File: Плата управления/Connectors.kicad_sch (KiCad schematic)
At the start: 9 parts, among them J1 Conn_02x10_Odd_Even, J11 Conn_02x07_Odd_Even, J2 CAN2, J3 CAN1, J4 A, J5 B, J6 C, J7 RS-485, J9 Conn_01x06

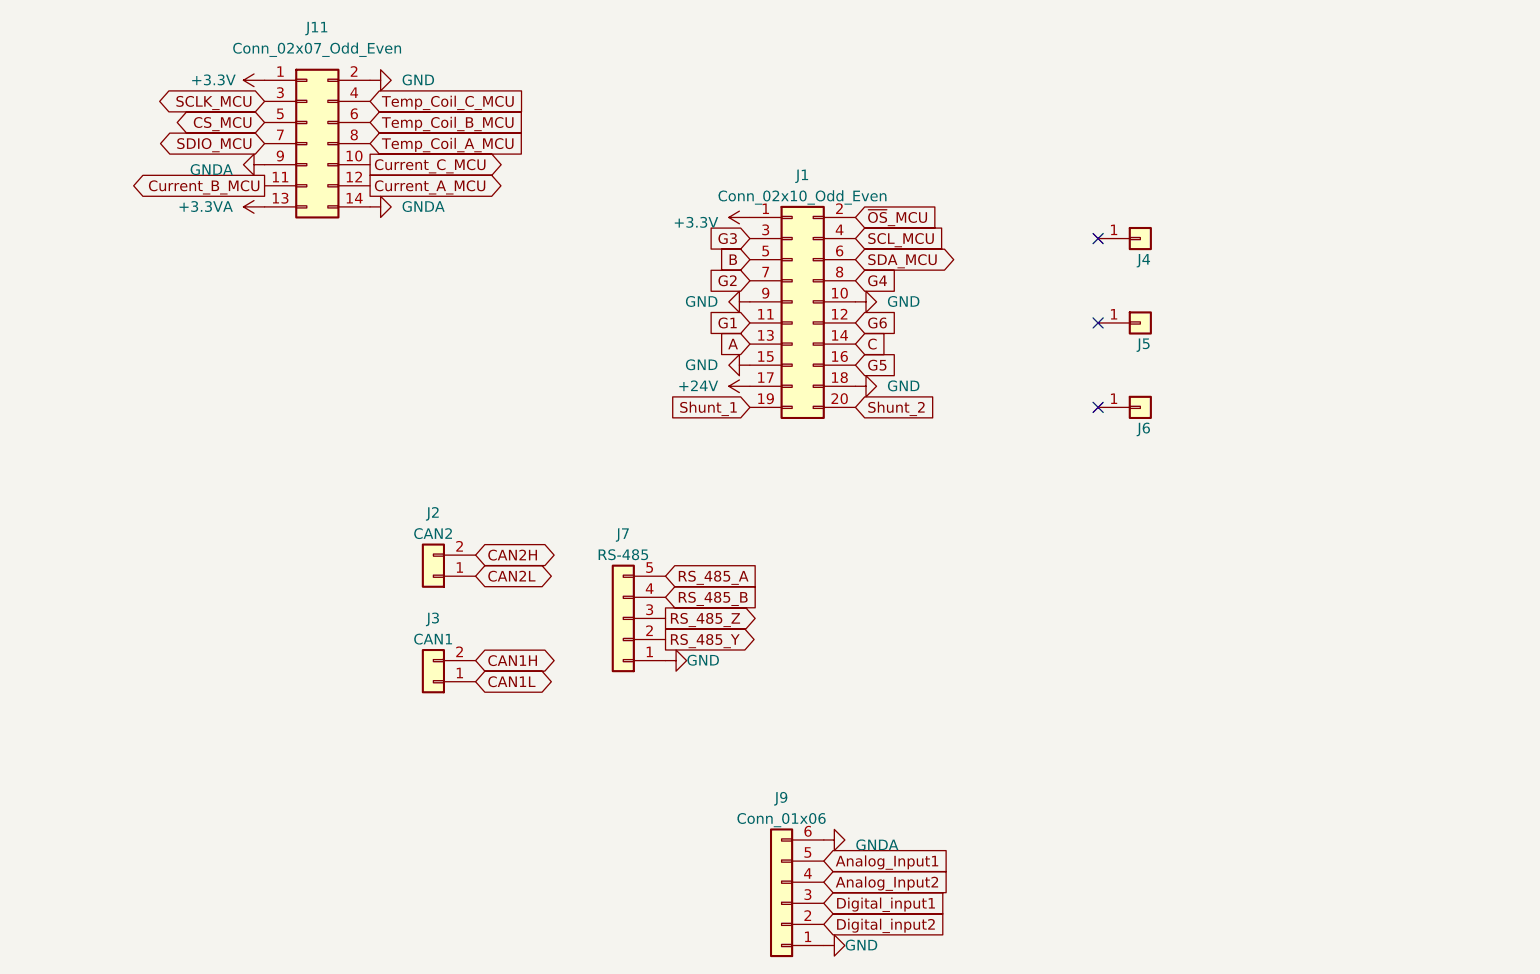
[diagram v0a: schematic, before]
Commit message: Редактировал схему
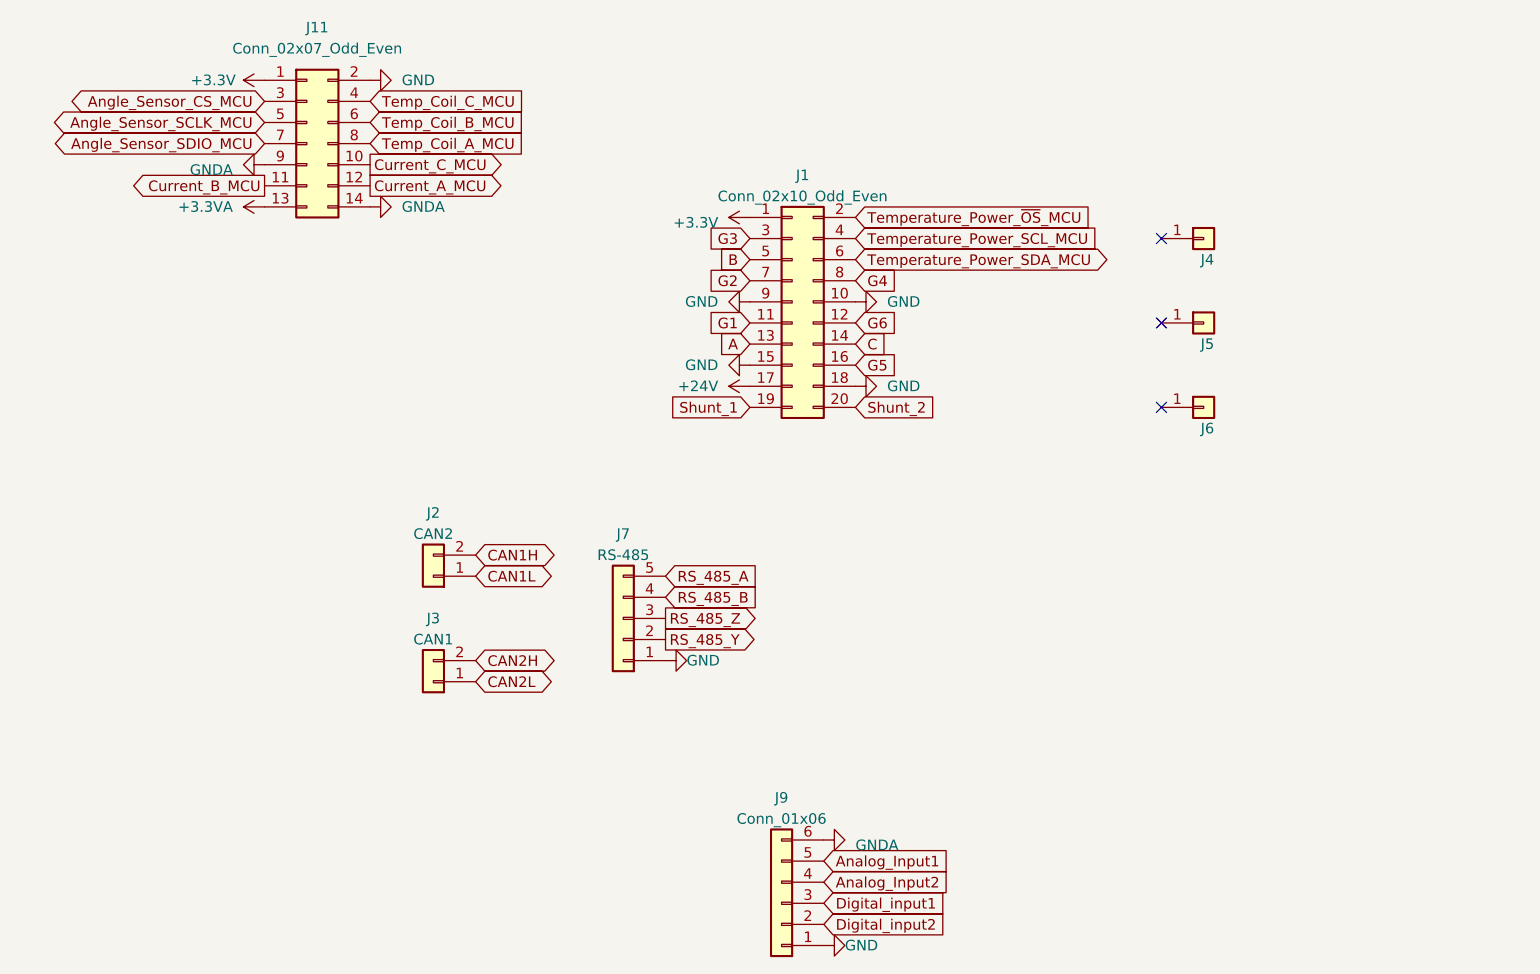
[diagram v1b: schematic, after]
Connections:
- net CAN1H: now also J2.2 (Pin_2); no longer J3.2 (Pin_2)
- net CAN1L: now also J2.1 (Pin_1); no longer J3.1 (Pin_1)
- net CAN2H: now also J3.2 (Pin_2); no longer J2.2 (Pin_2)
- net CAN2L: now also J3.1 (Pin_1); no longer J2.1 (Pin_1)
- net CS_MCU renamed Angle_Sensor_SCLK_MCU
- net SCLK_MCU renamed Angle_Sensor_CS_MCU
- net SCL_MCU renamed Temperature_Power_SCL_MCU
- net SDA_MCU renamed Temperature_Power_SDA_MCU
- net SDIO_MCU renamed Angle_Sensor_SDIO_MCU
- net ~{OS}_MCU renamed Temperature_Power_~{OS}_MCU
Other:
- moved on the sheet: J4, J5, J6

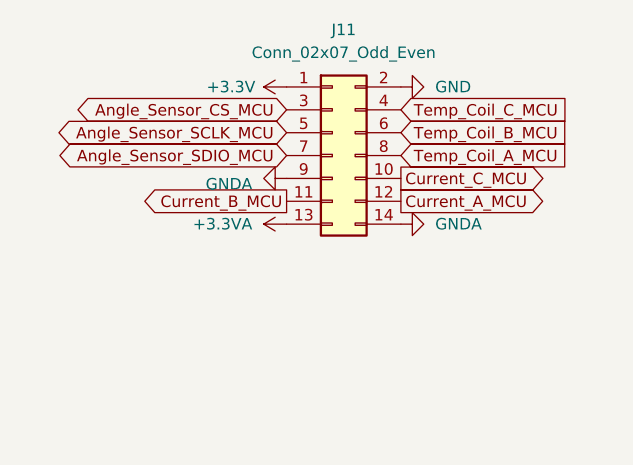
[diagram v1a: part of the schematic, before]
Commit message: Ещё нужно доработать
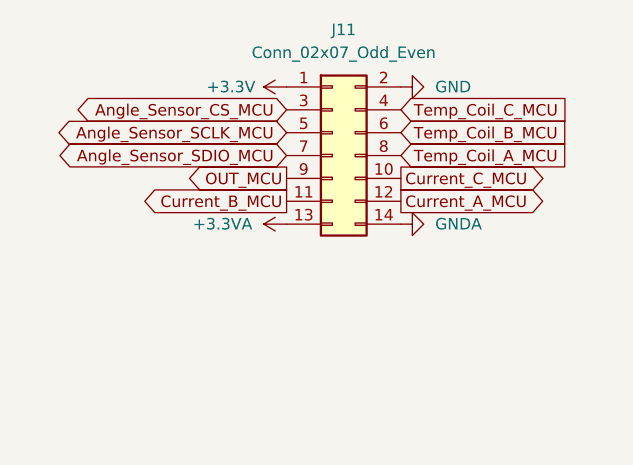
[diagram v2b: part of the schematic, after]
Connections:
- net GNDA: no longer J11.9 (Pin_9)
- new net OUT_MCU: J11.9 (Pin_9)
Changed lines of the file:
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@@
+    )
+  )
+  (global_label "OUT_MCU" (shape output) (at 91.44 69.85 180) (fields_autoplaced)
+    (effects (font (size 1.27 1.27)) (justify right))
+    (property "Intersheetrefs" "${INTERSHEET_REFS}" (at 79.8861 69.85 0)
+      (effects (font (size 1.27 1.27)) (justify right) hide)
     )
   )
@@
         )
       )
-    )
-  )
-  (symbol (lib_id "power:GNDA") (at 91.44 69.85 270) (unit 1)
-    (in_bom yes) (on_board yes) (dnp no) (fields_autoplaced)
-    (property "Reference" "#PWR037" (at 85.09 69.85 0)
-      (effects (font (size 1.27 1.27)) hide)
-    )
-    (property "Value" "GNDA" (at 87.63 70.485 90)
-      (effects (font (size 1.27 1.27)) (justify right))
-    )
-    (property "Footprint" "" (at 91.44 69.85 0)
-      (effects (font (size 1.27 1.27)) hide)
-    )
-    (property "Datasheet" "" (at 91.44 69.85 0)
-      (effects (font (size 1.27 1.27)) hide)
-    )
-    (pin "1")
-    (instances
-      (project "Плата управления"
-        (path "/75f4c67c-bbde-4446-8f82-67797a1b269f/f5e732cc-be4b-4207-bf28-0691ff32221d"
-          (reference "#PWR037") (unit 1)
-        )
-      )

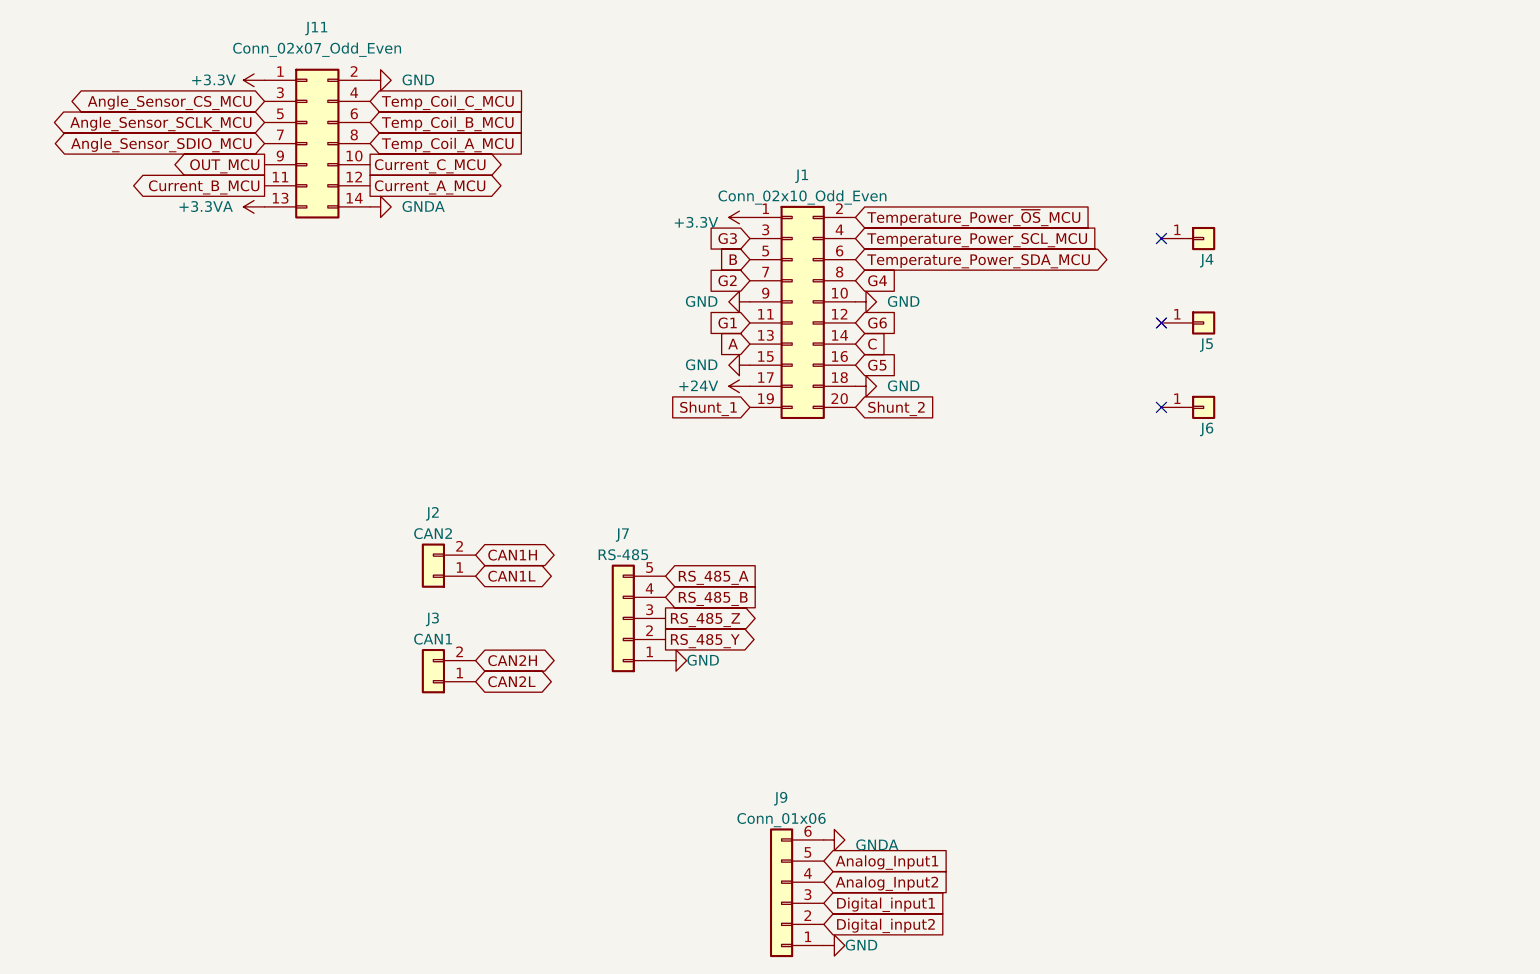
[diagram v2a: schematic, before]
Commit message: Добавил документы
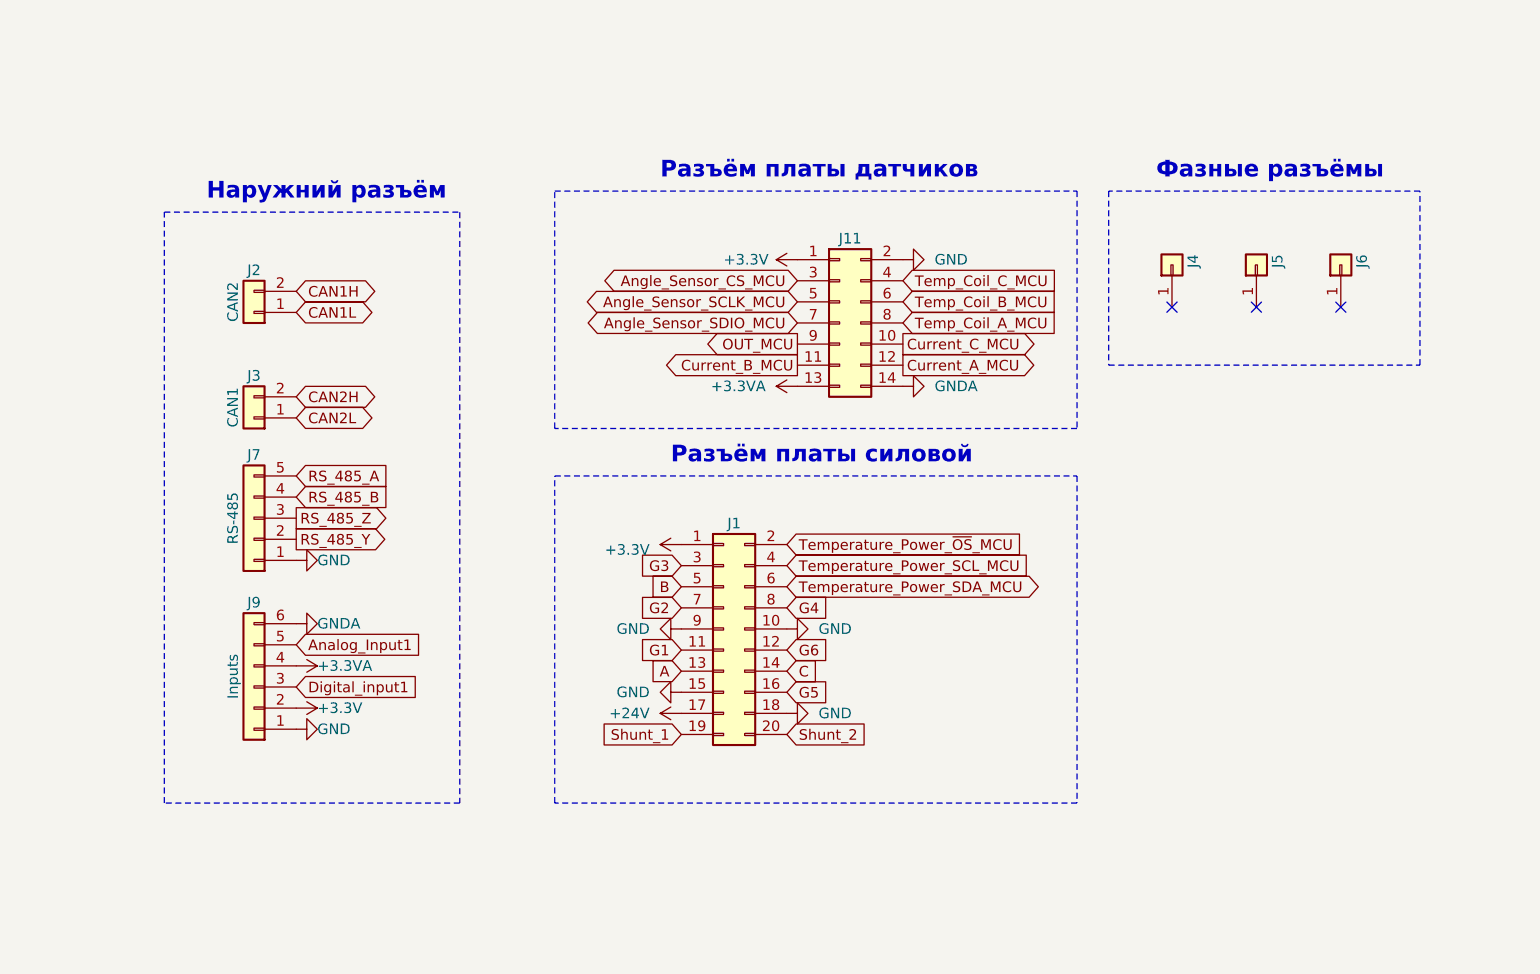
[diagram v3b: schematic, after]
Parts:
- J9: value Conn_01x06 -> Inputs
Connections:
- net Analog_Input2 is gone; now on net +3.3VA: J9.4 (Pin_4)
- net Digital_input2 is gone; now on net +3.3V: J9.2 (Pin_2)
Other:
- note added: "Наружний разъём"
- note added: "Разъём платы датчиков"
- note added: "Разъём платы силовой"
- note added: "Фазные разъёмы"
- moved on the sheet: J1, J11, J2, J3, J4, J5, J6, J7, J9
